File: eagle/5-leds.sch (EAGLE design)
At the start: 36 parts, among them T1 BC547, T10 BC547, T2 BC547, T3 BC547, T4 BC547, T5 BC547, T6 BC547, T7 BC547, T8 BC547, T9 BC547

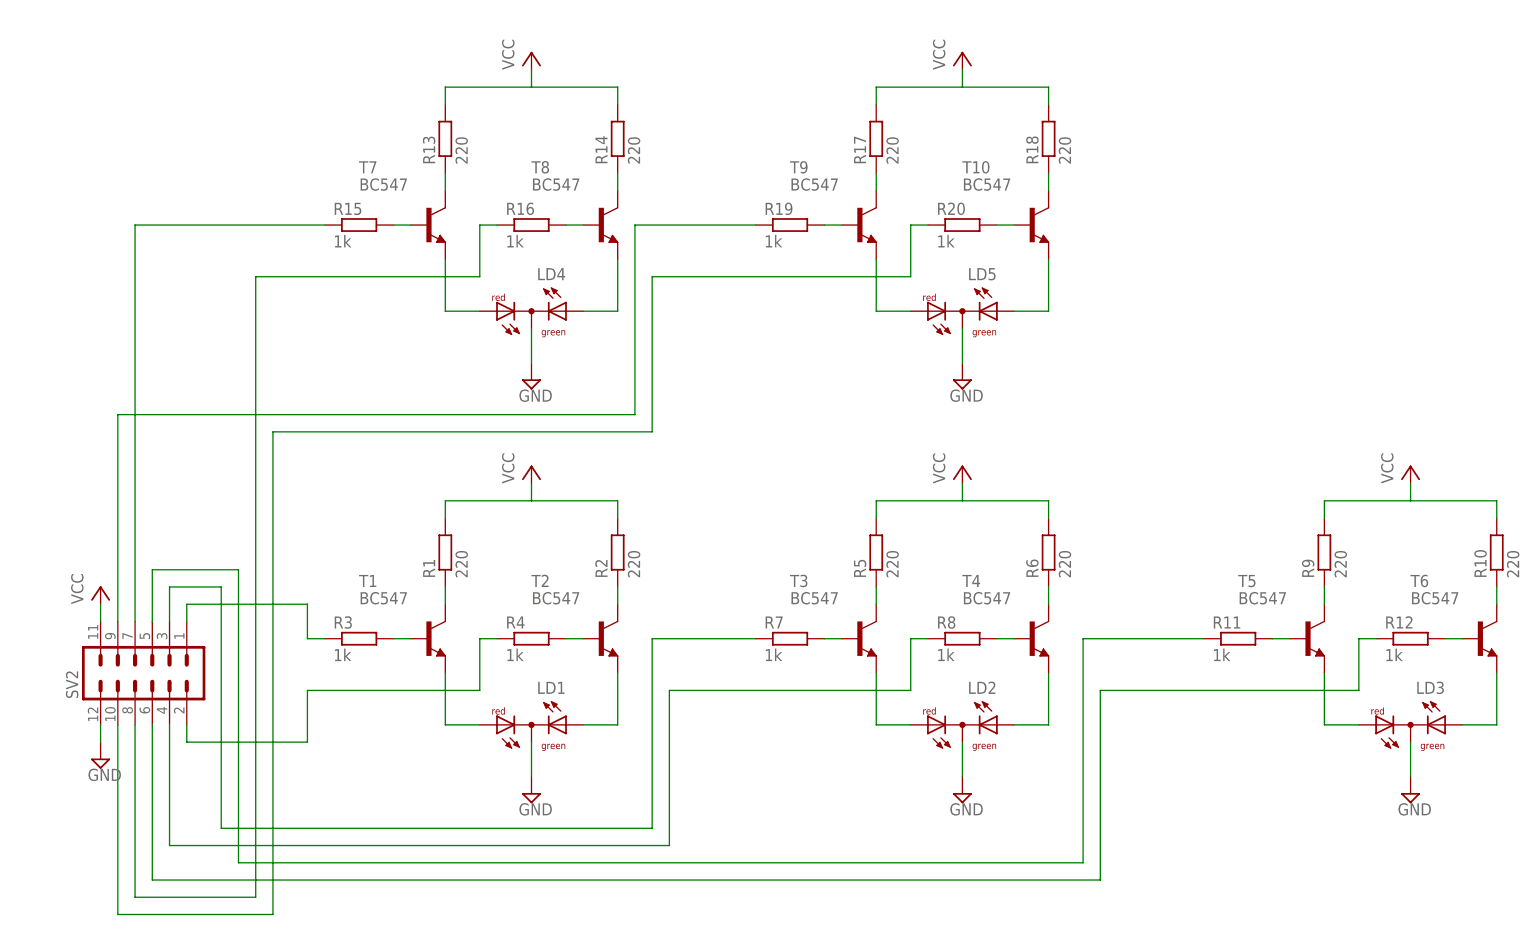
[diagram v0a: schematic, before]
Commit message: Tweak schematic, design board
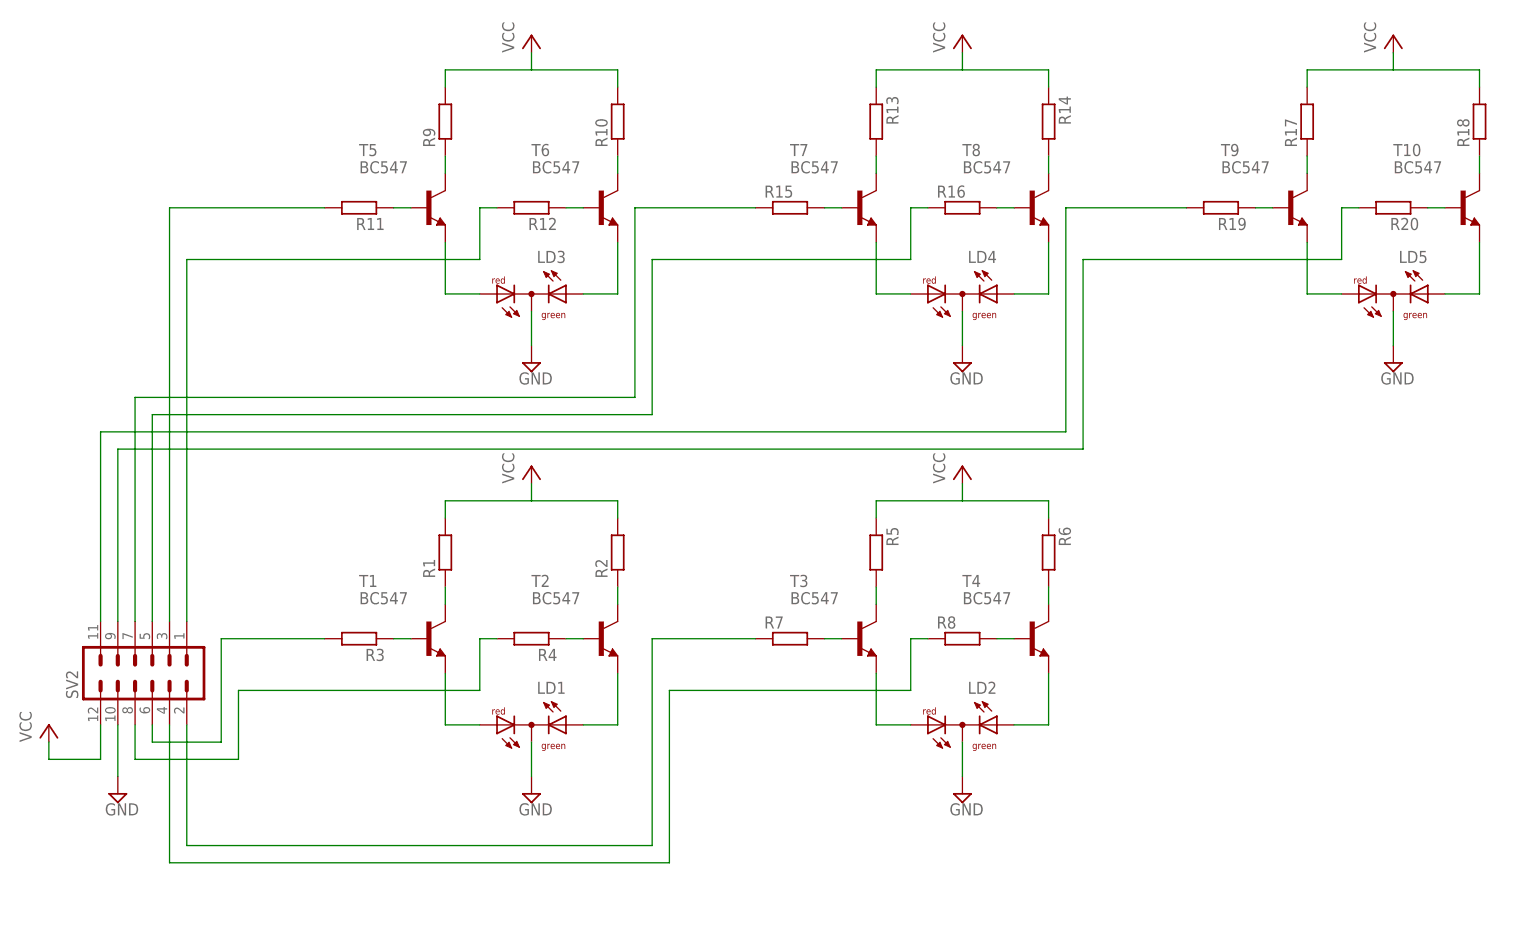
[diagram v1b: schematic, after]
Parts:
- R1, R10, R13, R14, R17, R18, R2, R5, R6, R9: value 220 -> (none); device rcl:R-EU_0207/10 -> rcl:R-EU_0207/7
- R11, R12, R15, R16, R19, R20, R3, R4, R7, R8: value 1k -> (none); device rcl:R-EU_0207/10 -> rcl:R-EU_0207/7
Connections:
- net GND: now also SV2.10; no longer SV2.12
- net N$13: now also R5.2; no longer R5.1
- net N$14: now also R6.2; no longer R6.1
- net N$17: now also SV2.2; no longer SV2.3
- net N$20: now also R12.2, SV2.1; no longer R12.1, SV2.6
- net N$23: now also R11.1; no longer R11.2
- net N$24: now also R12.1; no longer R12.2
- net N$25: now also R11.2, SV2.3; no longer R11.1, SV2.5
- net N$28: now also SV2.5; no longer SV2.8
- net N$29: now also R13.2; no longer R13.1
- net N$3: now also R3.1; no longer R3.2
- net N$30: now also R14.2; no longer R14.1
- net N$36: now also R20.2, SV2.9; no longer R20.1, SV2.10
- net N$39: now also R19.1; no longer R19.2
- net N$4: now also R4.1; no longer R4.2
- net N$40: now also R20.1; no longer R20.2
- net N$41: now also R19.2, SV2.11; no longer R19.1, SV2.9
- net N$5: now also R4.2, SV2.8; no longer R4.1, SV2.2
- net N$6: now also R3.2, SV2.6; no longer R3.1, SV2.1
- net VCC: now also R13.1, R14.1, R5.1, R6.1, SV2.12; no longer R13.2, R14.2, R5.2, R6.2, SV2.11
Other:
- moved on the sheet: LD3, LD4, LD5, R10, R11, R12, R13, R14, R15, R16, R17, R18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
